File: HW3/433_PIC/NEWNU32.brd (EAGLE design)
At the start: 50 x 50 mm, 22 parts, among them J1 USB-MB-H

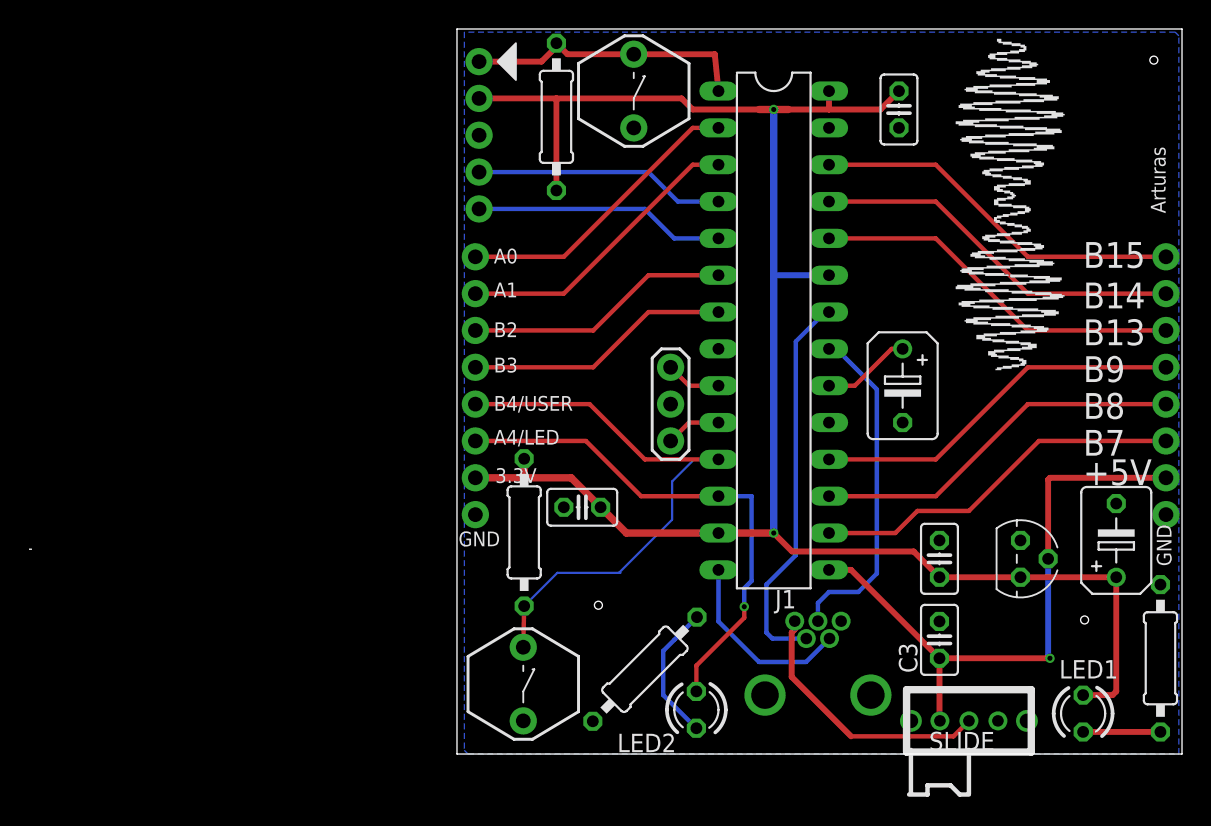
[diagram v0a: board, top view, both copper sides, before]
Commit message: Finished Initial Board
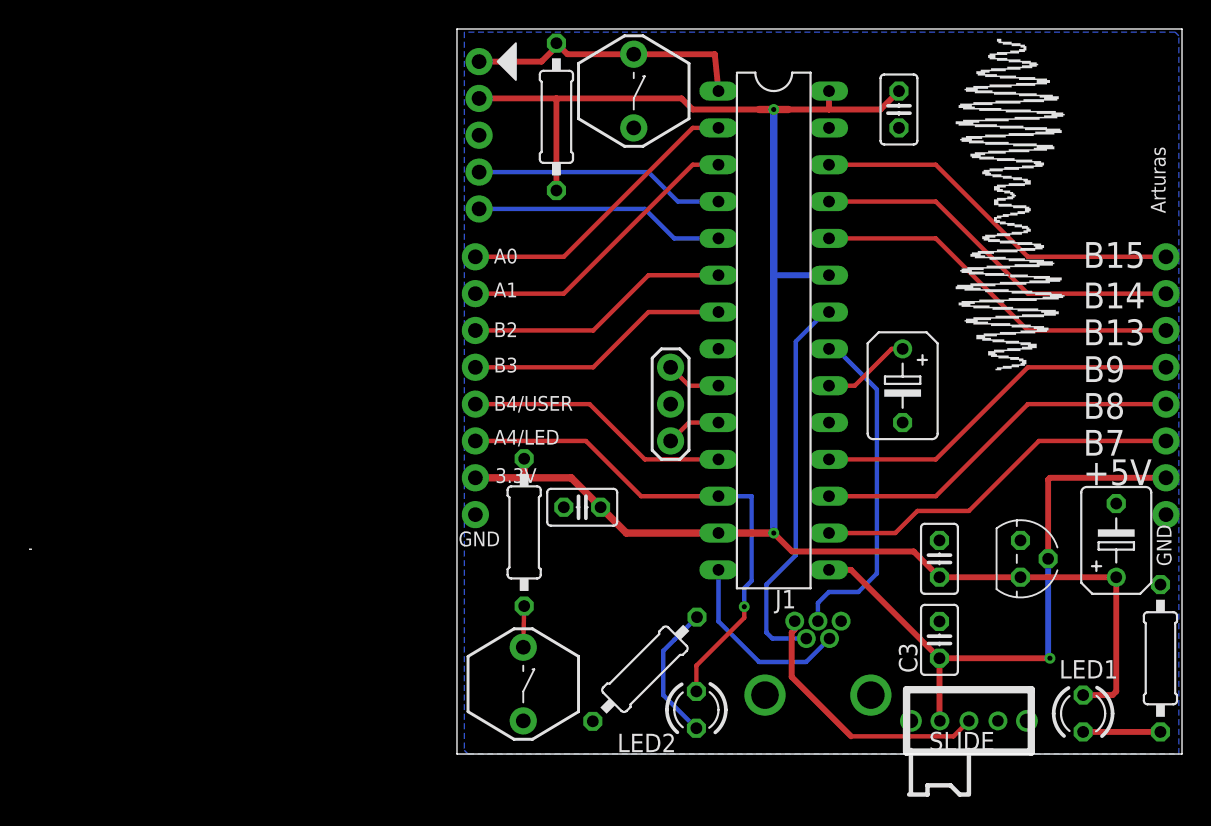
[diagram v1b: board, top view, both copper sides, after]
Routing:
- net B4/USER: track 40.4 -> 21.2 mm
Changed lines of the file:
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@@
 <text x="8.2296" y="18.6944" size="1.016" layer="22" font="vector" rot="MR0">3.3V</text>
 <text x="2.6416" y="14.3256" size="1.016" layer="22" font="vector" rot="MR0">GND</text>
-<hole x="9.7536" y="10.2616" drill="0.55"/>
-<hole x="43.2816" y="9.2456" drill="0.55"/>
-<hole x="48.0568" y="47.8536" drill="0.55"/>
 </plain>
 <attributes>
@@
 </class>
 </classes>
-<designrules name="SeeedStudio_2layer_DRU_no_angle_20140221">
+<designrules name="default">
 <description language="de">&lt;b&gt;EAGLE Design Rules&lt;/b&gt;
 &lt;p&gt;
@@
 necessary adjustments and save your customized
 design rules under a new name.</description>
-<description language="zh">&lt;b&gt;Seeed Studio EAGLE Design Rules&lt;/b&gt;
-</description>
 <param name="layerSetup" value="(1*16)"/>
-<param name="mtCopper" value="0.035mm 0.0175mm 0.035mm 0.035mm 0.035mm 0.035mm 0.035mm 0.035mm 0.035mm 0.035mm 0.035mm 0.035mm 0.035mm 0.035mm 0.0175mm 0.035mm"/>
-<param name="mtIsolate" value="1.5mm 1.1mm 0.2mm 0.15mm 0.2mm 0.15mm 0.2mm 0.15mm 0.2mm 0.15mm 0.2mm 0.15mm 0.2mm 0.15mm 0.2mm"/>
+<param name="mtCopper" value="0.035mm 0.035mm 0.035mm 0.035mm 0.035mm 0.035mm 0.035mm 0.035mm 0.035mm 0.035mm 0.035mm 0.035mm 0.035mm 0.035mm 0.035mm 0.035mm"/>
+<param name="mtIsolate" value="1.5mm 0.15mm 0.2mm 0.15mm 0.2mm 0.15mm 0.2mm 0.15mm 0.2mm 0.15mm 0.2mm 0.15mm 0.2mm 0.15mm 0.2mm"/>
 <param name="mdWireWire" value="6mil"/>
 <param name="mdWirePad" value="6mil"/>
@@
 <param name="mdPadVia" value="6mil"/>
 <param name="mdViaVia" value="6mil"/>
-<param name="mdSmdPad" value="0mil"/>
-<param name="mdSmdVia" value="0mil"/>
-<param name="mdSmdSmd" value="0mil"/>
-<param name="mdViaViaSameLayer" value="8mil"/>
+<param name="mdSmdPad" value="6mil"/>
+<param name="mdSmdVia" value="6mil"/>
+<param name="mdSmdSmd" value="6mil"/>
+<param name="mdViaViaSameLayer" value="6mil"/>
 <param name="mnLayersViaInSmd" value="2"/>
-<param name="mdCopperDimension" value="10mil"/>
-<param name="mdDrill" value="10mil"/>
+<param name="mdCopperDimension" value="40mil"/>
+<param name="mdDrill" value="6mil"/>
 <param name="mdSmdStop" value="0mil"/>
 <param name="msWidth" value="6mil"/>
-<param name="msDrill" value="12mil"/>
-<param name="msMicroVia" value="12mil"/>
+<param name="msDrill" value="0.35mm"/>
+<param name="msMicroVia" value="9.99mm"/>
 <param name="msBlindViaRatio" value="0.5"/>
 <param name="rvPadTop" value="0.25"/>
@@
 <param name="rlMinPadBottom" value="10mil"/>
 <param name="rlMaxPadBottom" value="20mil"/>
-<param name="rlMinViaOuter" value="6mil"/>
+<param name="rlMinViaOuter" value="8mil"/>
 <param name="rlMaxViaOuter" value="20mil"/>
-<param name="rlMinViaInner" value="6mil"/>
+<param name="rlMinViaInner" value="8mil"/>
 <param name="rlMaxViaInner" value="20mil"/>
 <param name="rlMinMicroViaOuter" value="4mil"/>
@@
 <param name="psTop" value="-1"/>
 <param name="psBottom" value="-1"/>
-<param name="psFirst" value="0"/>
+<param name="psFirst" value="-1"/>
 <param name="psElongationLong" value="100"/>
 <param name="psElongationOffset" value="100"/>
 <param name="mvStopFrame" value="1"/>
 <param name="mvCreamFrame" value="0"/>
-<param name="mlMinStopFrame" value="2mil"/>
-<param name="mlMaxStopFrame" value="2mil"/>
+<param name="mlMinStopFrame" value="4mil"/>
+<param name="mlMaxStopFrame" value="4mil"/>
 <param name="mlMinCreamFrame" value="0mil"/>
 <param name="mlMaxCreamFrame" value="0mil"/>
-<param name="mlViaStopLimit" value="100mil"/>
+<param name="mlViaStopLimit" value="0mil"/>
 <param name="srRoundness" value="0"/>
 <param name="srMinRoundness" value="0mil"/>
@@
 <param name="checkAngle" value="0"/>
 <param name="checkFont" value="1"/>
-<param name="checkRestrict" value="0"/>
+<param name="checkRestrict" value="1"/>
 <param name="checkStop" value="0"/>
 <param name="checkValues" value="0"/>
@@
 <vertex x="49.53" y="49.784"/>
 </polygon>
-<wire x1="25.654" y1="22.86" x2="30.734" y2="22.86" width="0" layer="19" extent="1-1"/>
+<wire x1="30.734" y1="22.86" x2="25.654" y2="22.86" width="0" layer="19" extent="1-1"/>
 </signal>
 <signal name="+5V">
@@
 <wire x1="9.144" y1="24.13" x2="12.954" y2="20.32" width="0.3048" layer="1"/>
 <wire x1="12.954" y1="20.32" x2="18.034" y2="20.32" width="0.3048" layer="1"/>
-<wire x1="4.633628125" y1="10.203578125" x2="6.92685" y2="12.4968" width="0.1524" layer="16"/>
-<wire x1="6.92685" y1="12.4968" x2="11.176" y2="12.4968" width="0.1524" layer="16"/>
-<wire x1="11.176" y1="12.4968" x2="11.2776" y2="12.4968" width="0.1524" layer="16"/>
-<wire x1="11.176" y1="12.4968" x2="14.8336" y2="16.1544" width="0.1524" layer="16"/>
-<wire x1="14.8336" y1="16.1544" x2="14.8336" y2="18.796" width="0.1524" layer="16"/>
-<wire x1="14.8336" y1="18.796" x2="16.3576" y2="20.32" width="0.1524" layer="16"/>
-<wire x1="16.3576" y1="20.32" x2="18.034" y2="20.32" width="0.1524" layer="16"/>
+<wire x1="4.633628125" y1="10.203578125" x2="12.954" y2="20.32" width="0" layer="19" extent="1-1"/>
 </signal>
 <signal name="A4/LED">

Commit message: Built HW1 Circuit and Began Code
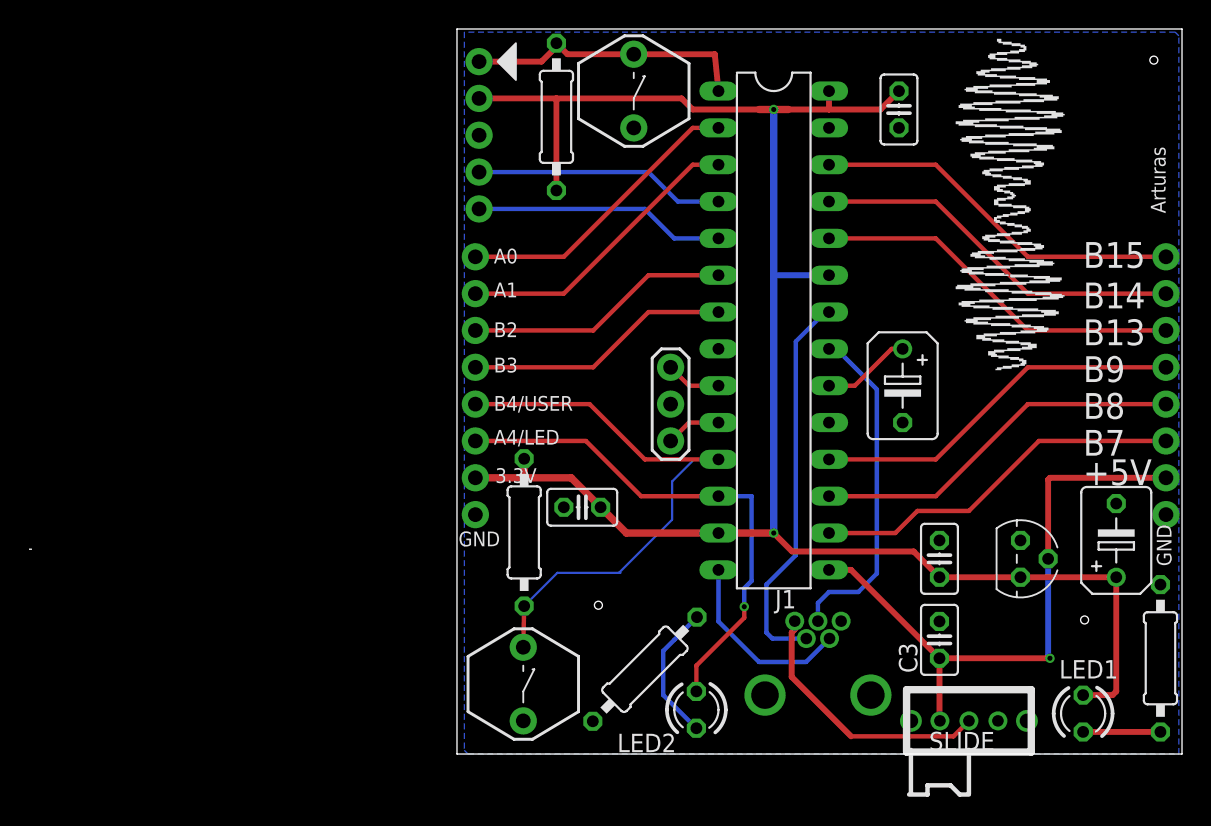
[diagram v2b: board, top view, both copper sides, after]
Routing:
- net B4/USER: track 21.2 -> 40.4 mm
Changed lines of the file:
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@@
 <text x="8.2296" y="18.6944" size="1.016" layer="22" font="vector" rot="MR0">3.3V</text>
 <text x="2.6416" y="14.3256" size="1.016" layer="22" font="vector" rot="MR0">GND</text>
+<hole x="9.7536" y="10.2616" drill="0.55"/>
+<hole x="43.2816" y="9.2456" drill="0.55"/>
+<hole x="48.0568" y="47.8536" drill="0.55"/>
 </plain>
 <attributes>
@@
 </class>
 </classes>
-<designrules name="default">
+<designrules name="SeeedStudio_2layer_DRU_no_angle_20140221">
 <description language="de">&lt;b&gt;EAGLE Design Rules&lt;/b&gt;
 &lt;p&gt;
@@
 necessary adjustments and save your customized
 design rules under a new name.</description>
+<description language="zh">&lt;b&gt;Seeed Studio EAGLE Design Rules&lt;/b&gt;
+</description>
 <param name="layerSetup" value="(1*16)"/>
-<param name="mtCopper" value="0.035mm 0.035mm 0.035mm 0.035mm 0.035mm 0.035mm 0.035mm 0.035mm 0.035mm 0.035mm 0.035mm 0.035mm 0.035mm 0.035mm 0.035mm 0.035mm"/>
-<param name="mtIsolate" value="1.5mm 0.15mm 0.2mm 0.15mm 0.2mm 0.15mm 0.2mm 0.15mm 0.2mm 0.15mm 0.2mm 0.15mm 0.2mm 0.15mm 0.2mm"/>
+<param name="mtCopper" value="0.035mm 0.0175mm 0.035mm 0.035mm 0.035mm 0.035mm 0.035mm 0.035mm 0.035mm 0.035mm 0.035mm 0.035mm 0.035mm 0.035mm 0.0175mm 0.035mm"/>
+<param name="mtIsolate" value="1.5mm 1.1mm 0.2mm 0.15mm 0.2mm 0.15mm 0.2mm 0.15mm 0.2mm 0.15mm 0.2mm 0.15mm 0.2mm 0.15mm 0.2mm"/>
 <param name="mdWireWire" value="6mil"/>
 <param name="mdWirePad" value="6mil"/>
@@
 <param name="mdPadVia" value="6mil"/>
 <param name="mdViaVia" value="6mil"/>
-<param name="mdSmdPad" value="6mil"/>
-<param name="mdSmdVia" value="6mil"/>
-<param name="mdSmdSmd" value="6mil"/>
-<param name="mdViaViaSameLayer" value="6mil"/>
+<param name="mdSmdPad" value="0mil"/>
+<param name="mdSmdVia" value="0mil"/>
+<param name="mdSmdSmd" value="0mil"/>
+<param name="mdViaViaSameLayer" value="8mil"/>
 <param name="mnLayersViaInSmd" value="2"/>
-<param name="mdCopperDimension" value="40mil"/>
-<param name="mdDrill" value="6mil"/>
+<param name="mdCopperDimension" value="10mil"/>
+<param name="mdDrill" value="10mil"/>
 <param name="mdSmdStop" value="0mil"/>
 <param name="msWidth" value="6mil"/>
-<param name="msDrill" value="0.35mm"/>
-<param name="msMicroVia" value="9.99mm"/>
+<param name="msDrill" value="12mil"/>
+<param name="msMicroVia" value="12mil"/>
 <param name="msBlindViaRatio" value="0.5"/>
 <param name="rvPadTop" value="0.25"/>
@@
 <param name="rlMinPadBottom" value="10mil"/>
 <param name="rlMaxPadBottom" value="20mil"/>
-<param name="rlMinViaOuter" value="8mil"/>
+<param name="rlMinViaOuter" value="6mil"/>
 <param name="rlMaxViaOuter" value="20mil"/>
-<param name="rlMinViaInner" value="8mil"/>
+<param name="rlMinViaInner" value="6mil"/>
 <param name="rlMaxViaInner" value="20mil"/>
 <param name="rlMinMicroViaOuter" value="4mil"/>
@@
 <param name="psTop" value="-1"/>
 <param name="psBottom" value="-1"/>
-<param name="psFirst" value="-1"/>
+<param name="psFirst" value="0"/>
 <param name="psElongationLong" value="100"/>
 <param name="psElongationOffset" value="100"/>
 <param name="mvStopFrame" value="1"/>
 <param name="mvCreamFrame" value="0"/>
-<param name="mlMinStopFrame" value="4mil"/>
-<param name="mlMaxStopFrame" value="4mil"/>
+<param name="mlMinStopFrame" value="2mil"/>
+<param name="mlMaxStopFrame" value="2mil"/>
 <param name="mlMinCreamFrame" value="0mil"/>
 <param name="mlMaxCreamFrame" value="0mil"/>
-<param name="mlViaStopLimit" value="0mil"/>
+<param name="mlViaStopLimit" value="100mil"/>
 <param name="srRoundness" value="0"/>
 <param name="srMinRoundness" value="0mil"/>
@@
 <param name="checkAngle" value="0"/>
 <param name="checkFont" value="1"/>
-<param name="checkRestrict" value="1"/>
+<param name="checkRestrict" value="0"/>
 <param name="checkStop" value="0"/>
 <param name="checkValues" value="0"/>
@@
 <vertex x="49.53" y="49.784"/>
 </polygon>
-<wire x1="30.734" y1="22.86" x2="25.654" y2="22.86" width="0" layer="19" extent="1-1"/>
+<wire x1="25.654" y1="22.86" x2="30.734" y2="22.86" width="0" layer="19" extent="1-1"/>
 </signal>
 <signal name="+5V">
@@
 <wire x1="9.144" y1="24.13" x2="12.954" y2="20.32" width="0.3048" layer="1"/>
 <wire x1="12.954" y1="20.32" x2="18.034" y2="20.32" width="0.3048" layer="1"/>
-<wire x1="4.633628125" y1="10.203578125" x2="12.954" y2="20.32" width="0" layer="19" extent="1-1"/>
+<wire x1="4.633628125" y1="10.203578125" x2="6.92685" y2="12.4968" width="0.1524" layer="16"/>
+<wire x1="6.92685" y1="12.4968" x2="11.176" y2="12.4968" width="0.1524" layer="16"/>
+<wire x1="11.176" y1="12.4968" x2="11.2776" y2="12.4968" width="0.1524" layer="16"/>
+<wire x1="11.176" y1="12.4968" x2="14.8336" y2="16.1544" width="0.1524" layer="16"/>
+<wire x1="14.8336" y1="16.1544" x2="14.8336" y2="18.796" width="0.1524" layer="16"/>
+<wire x1="14.8336" y1="18.796" x2="16.3576" y2="20.32" width="0.1524" layer="16"/>
+<wire x1="16.3576" y1="20.32" x2="18.034" y2="20.32" width="0.1524" layer="16"/>
 </signal>
 <signal name="A4/LED">
